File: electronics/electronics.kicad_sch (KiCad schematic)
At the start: 16 parts, among them J1 USB_C_Receptacle_USB2.0_16P, U1 ESP32-C6-WROOM-1, U2 AM2302, U3 LM3940IMP-3.3

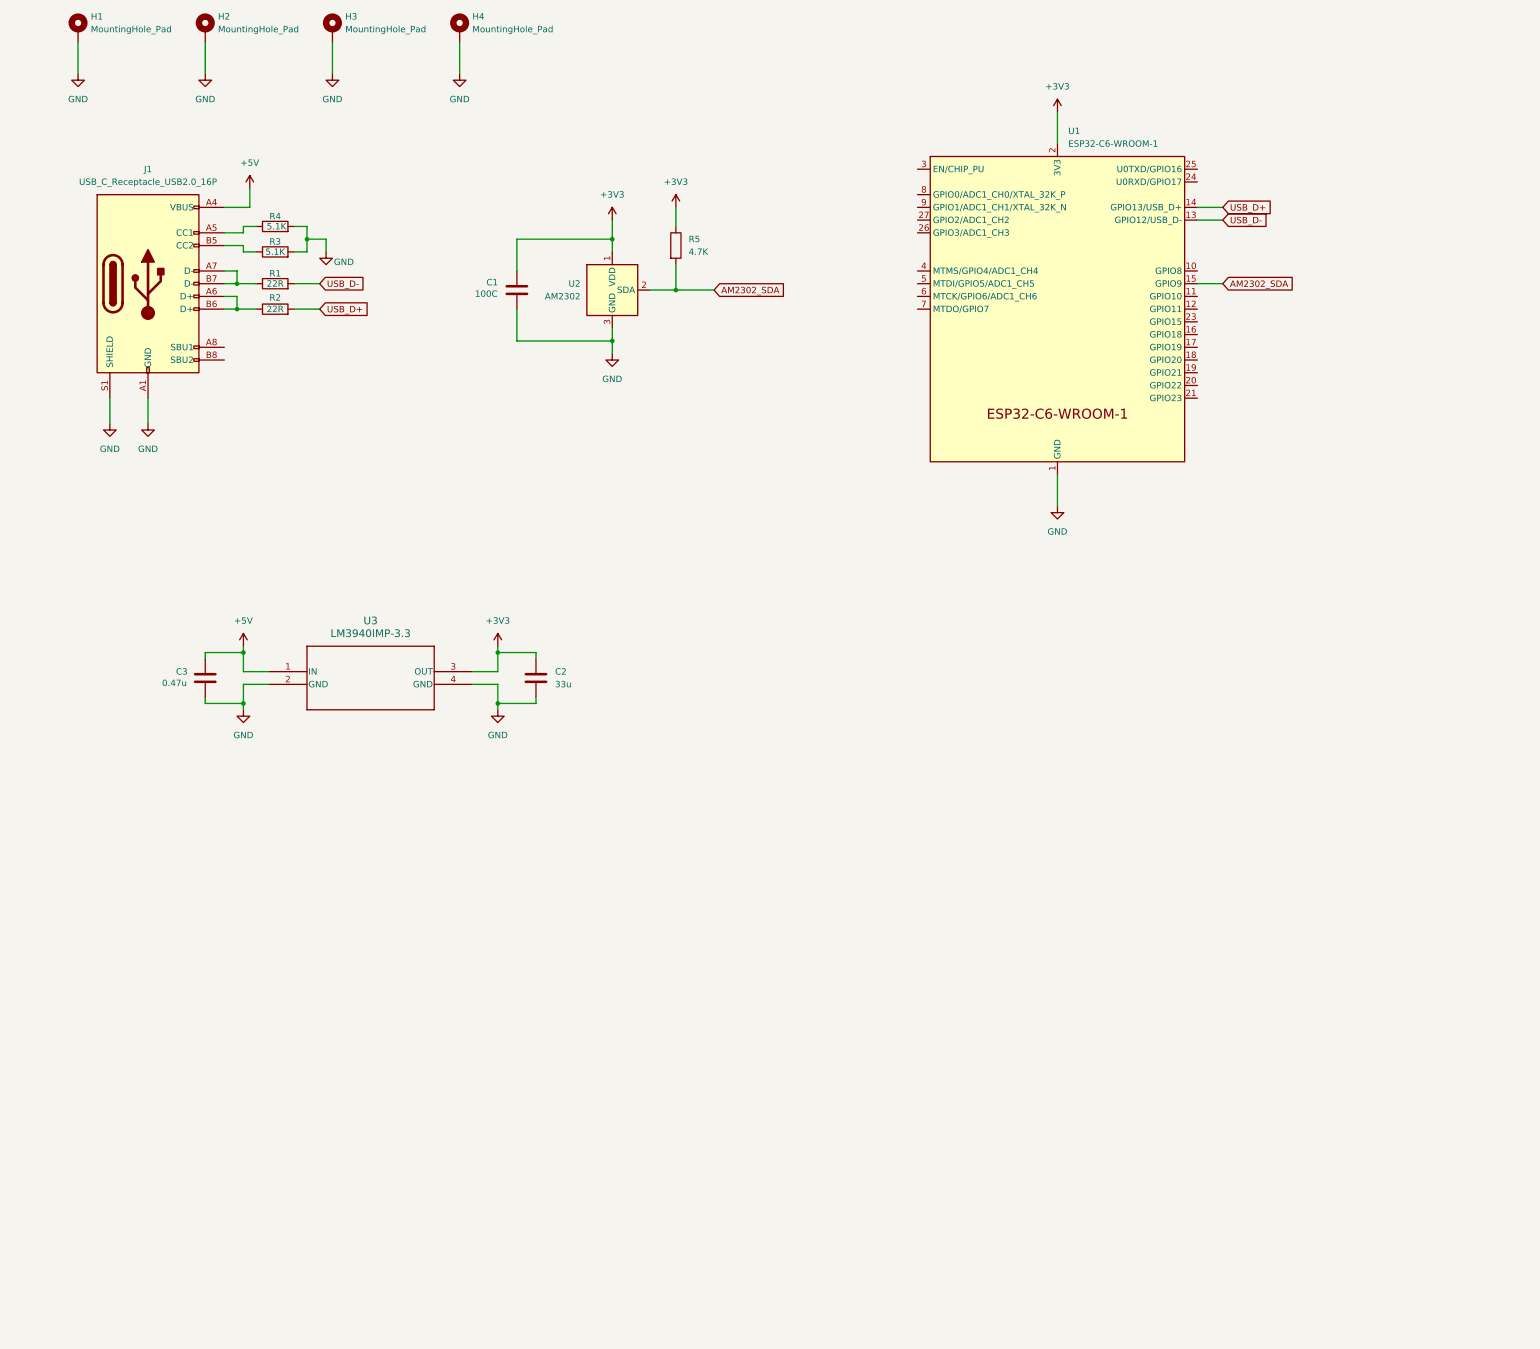
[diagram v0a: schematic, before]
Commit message: schematic: remade schematic
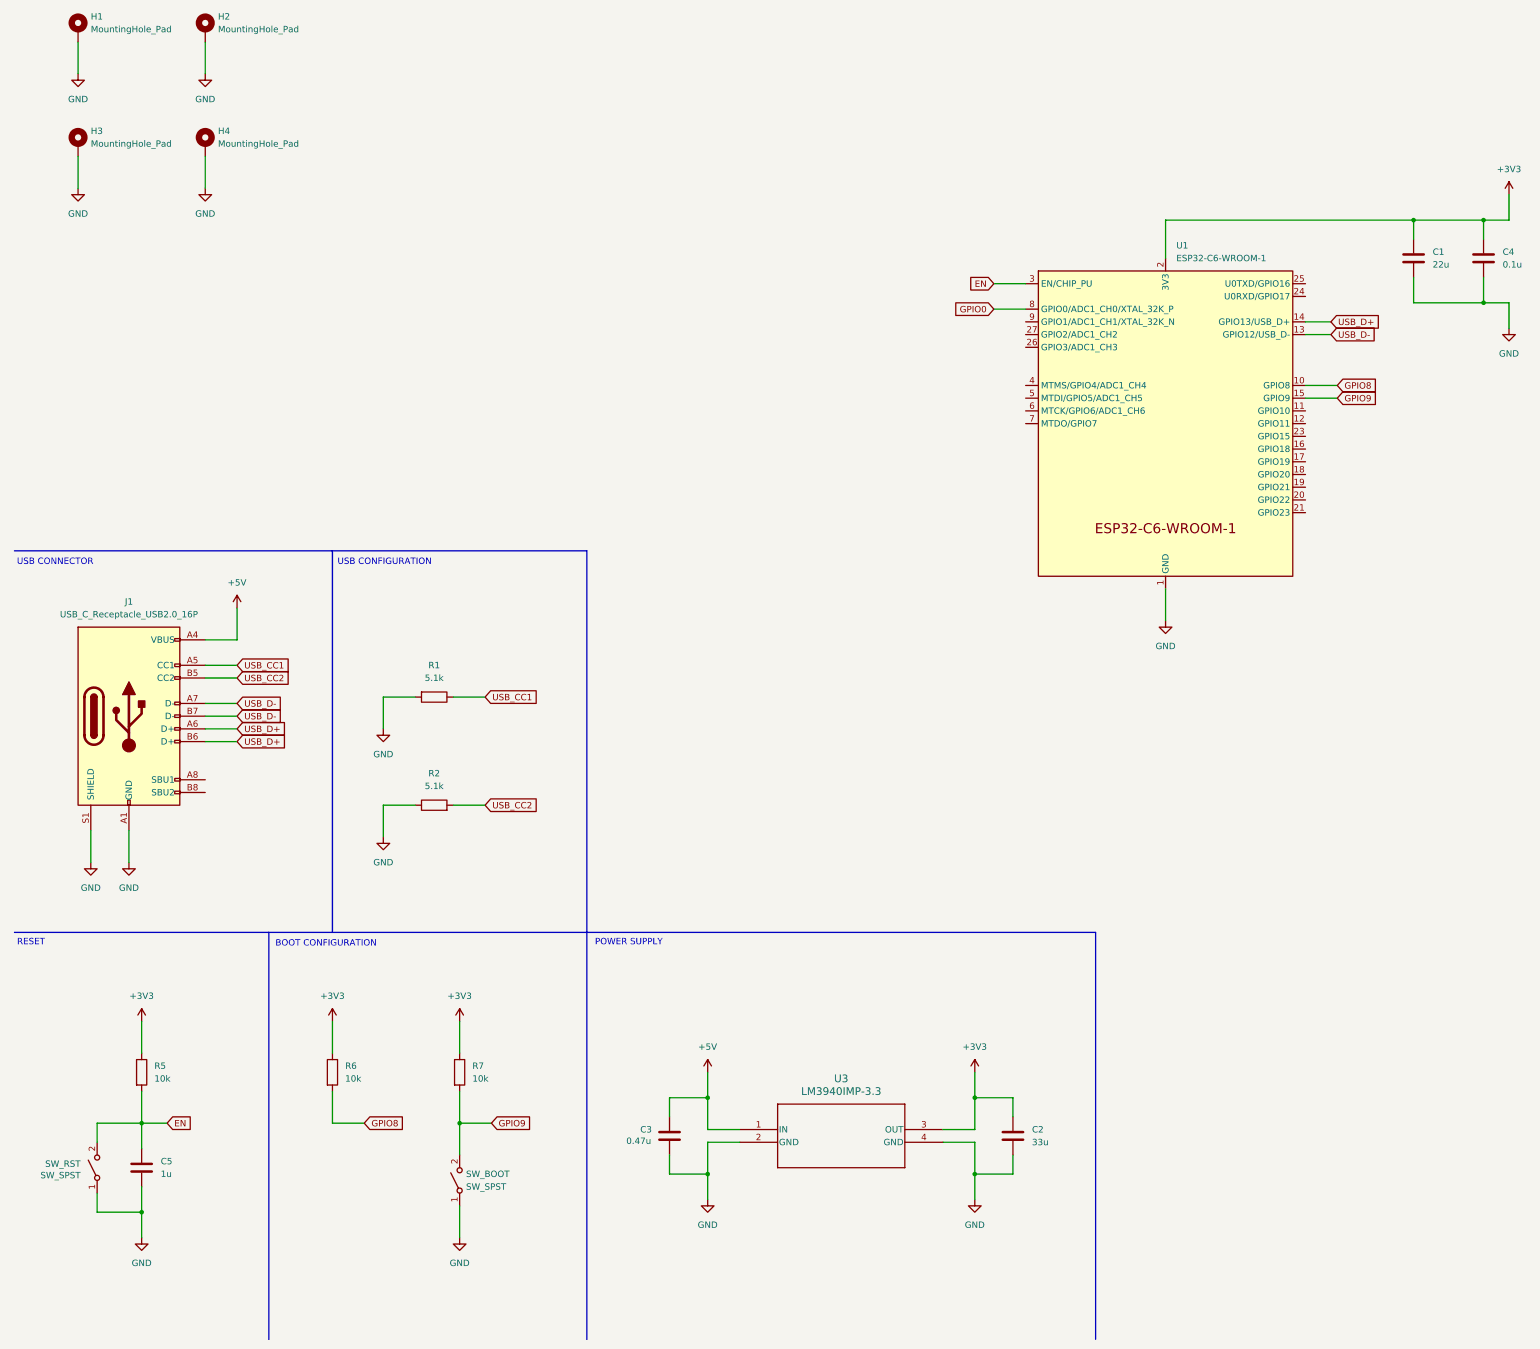
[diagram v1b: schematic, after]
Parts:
- removed R3, R4: 5.1K, Resistor_SMD:R_0805_2012Metric_Pad1.20x1.40mm_HandSolder, symbol Device:R
- removed U2: AM2302, Sensor:ASAIR_AM2302_P2.54mm_Lead2.75mm_TabDown, symbol Sensor:AM2302
- added C4: 0.1u, symbol Device:C
- added C5: 1u, Capacitor_SMD:C_0805_2012Metric_Pad1.18x1.45mm_HandSolder, symbol Device:C
- added R6, R7: 10k, Resistor_SMD:R_0805_2012Metric_Pad1.20x1.40mm_HandSolder, symbol Device:R
- added SW_BOOT, SW_RST: SW_SPST, symbol Switch:SW_SPST
- C1: value 100C -> 22u; footprint Capacitor_SMD:C_0805_2012Metric_Pad1.18x1.45mm_HandSolder -> (none)
- R1, R2: value 22R -> 5.1k; footprint Resistor_SMD:R_0805_2012Metric_Pad1.20x1.40mm_HandSolder -> (none)
- R5: value 4.7K -> 10k
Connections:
- net +3V3: now also C4.1, R6.1, R7.1
- net GND: now also R1.2, R2.1, C4.2, C5.2, SW_BOOT.1 (A), SW_RST.1 (A)
- net USB_D+: now also J1.A6 (D+), J1.B6 (D+); no longer R2.2
- net USB_D-: now also J1.A7 (D-), J1.B7 (D-); no longer R1.2
- net USB_CC1: now reaches J1.A5 (CC1)
- net USB_CC1: now also R1.1
- net USB_CC2: now reaches J1.B5 (CC2)
- net USB_CC2: now also R2.2
- net GPIO8: now reaches U1.10 (GPIO8)
- net GPIO8: now also R6.2
- net EN: now reaches U1.3 (EN/CHIP_PU)
- net EN: now also R5.2, C5.1, SW_RST.2 (B)
- net GPIO0: now reaches U1.8 (GPIO0/ADC1_CH0/XTAL_32K_P)
- net AM2302_SDA renamed GPIO9
- net GPIO9: now also R7.2, SW_BOOT.2 (B); no longer R5.2
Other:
- note added: "BOOT CONFIGURATION"
- note added: "POWER SUPPLY"
- note added: "RESET"
- note added: "USB CONFIGURATION"
- note added: "USB CONNECTOR"
- moved on the sheet: C2, C3, H3, H4, J1, U1, U3
